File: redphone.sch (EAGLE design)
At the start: 228 parts, among them IC1 EP4CE22U14I7N, IC10 MPU9250, IC11 PCA9633TK, IC12 BME280, IC13 W25Q64FV, IC14 MC-1010-G, IC15 MAX2659, IC2 STM32F429NI, IC20 MP34DT01, IC25 APDS-9960, IC3 MT48LC16M16A2B4, IC4 MT48LC16M16A2B4, IC5 W25Q64FV, IC6 SIM800H, IC7 TPS65217, IC8 ESP8266, IC9 WM8903, M1 VIBRO, Q1 IRLML2502, Q2 IRLML2502, Q3 IRLML2502, SW1 PWR, SW3 VOL+, SW4 VOL-, X1 USB, X2 OV5647, X3 RM68120_LCD, X4 MICRO_SIM_SDS8, X5 LG_P715_TS, X7 AUDIO-JACKSMD, X8 FPC_I9500_BAT_CON, Y1 2.4Ghz, Y3 2.4Ghz, Y4 GSM_PCB

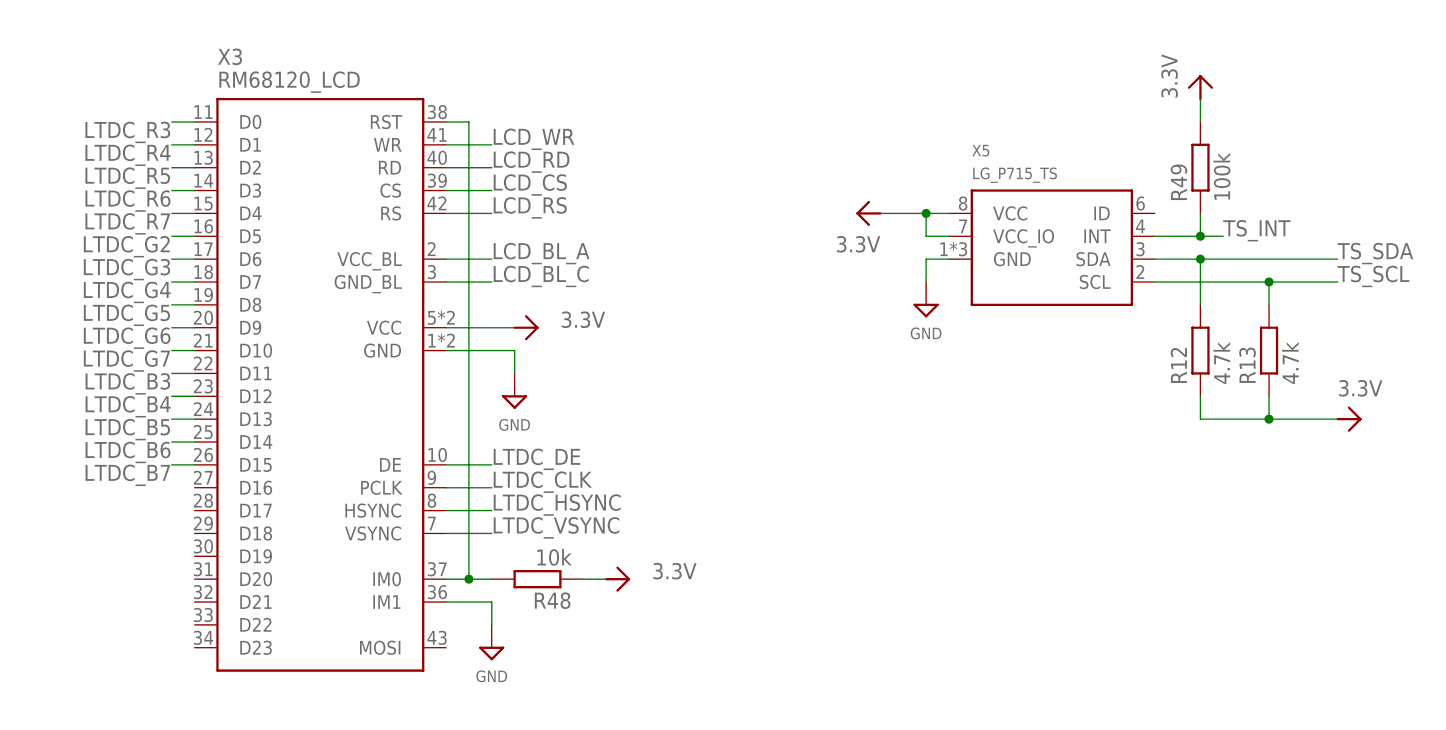
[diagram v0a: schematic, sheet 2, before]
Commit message: updeted LCD connector, connected 35 pin to GND
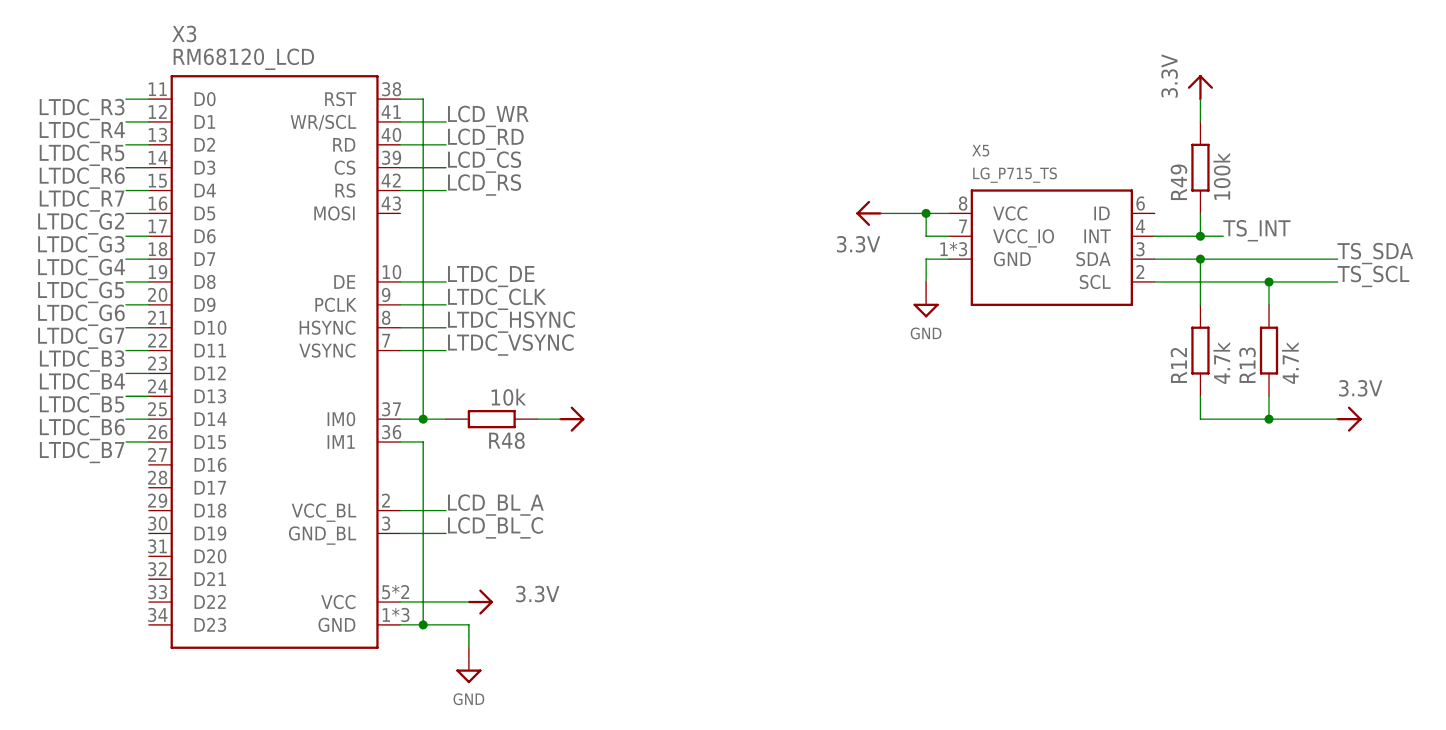
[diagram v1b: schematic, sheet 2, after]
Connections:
- net LCD_WR: now also X3.WR/SCL; no longer X3.WR
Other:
- moved on the sheet: R48, X3
